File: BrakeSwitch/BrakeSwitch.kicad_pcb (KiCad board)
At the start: 2 copper layers, 82.3 x 59.8 mm, 31 parts, among them J1 12V_in, J2 LightPlug, J2 Signal_Breakout, J3 5V_out, J4 Front_Loop, J5 Rear_Loop, J6 12V_Out, J7 Front_Brake_Switch, J8 Rear_Brake_Switch, J9 Light_In, Q1 NMOS, SW1 AT SW-R2-2B-F-1-0, U1 XL1509-5.0, U2 LMV321, U3 LMV321

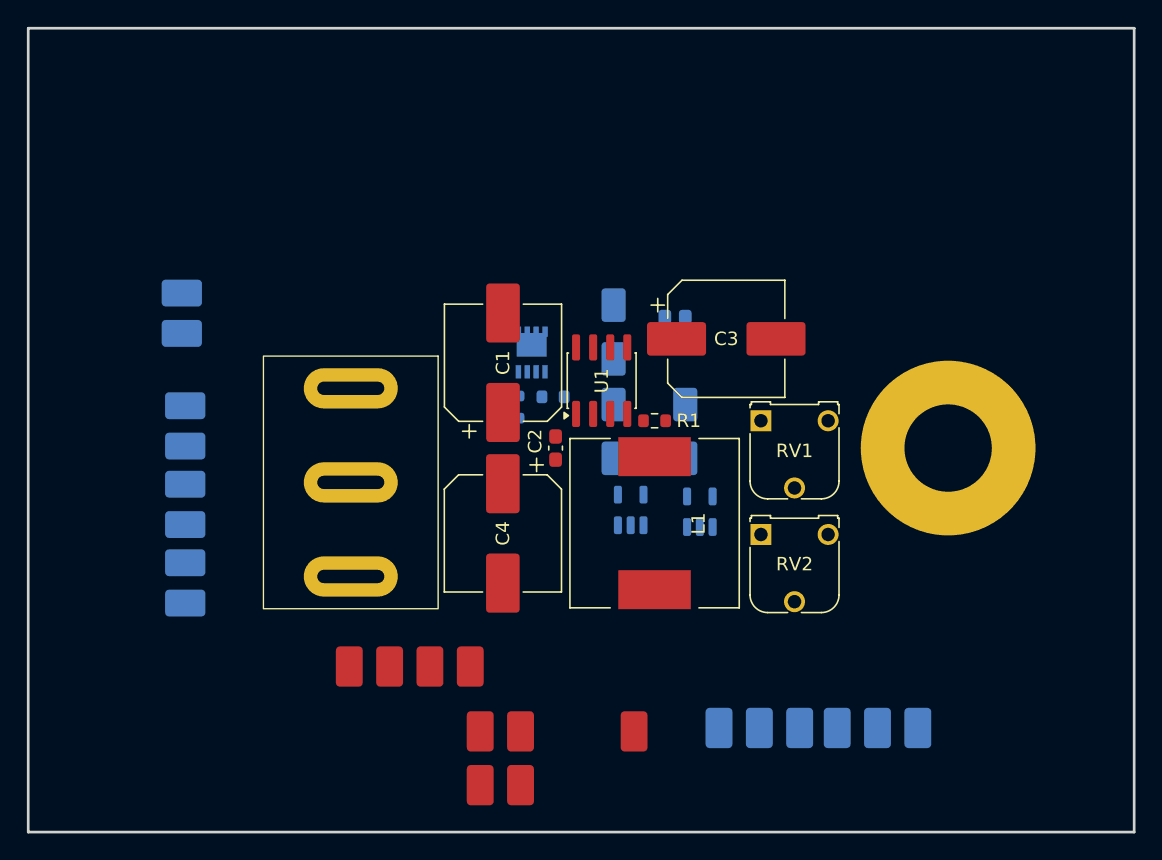
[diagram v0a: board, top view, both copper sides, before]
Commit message: Layout doneish
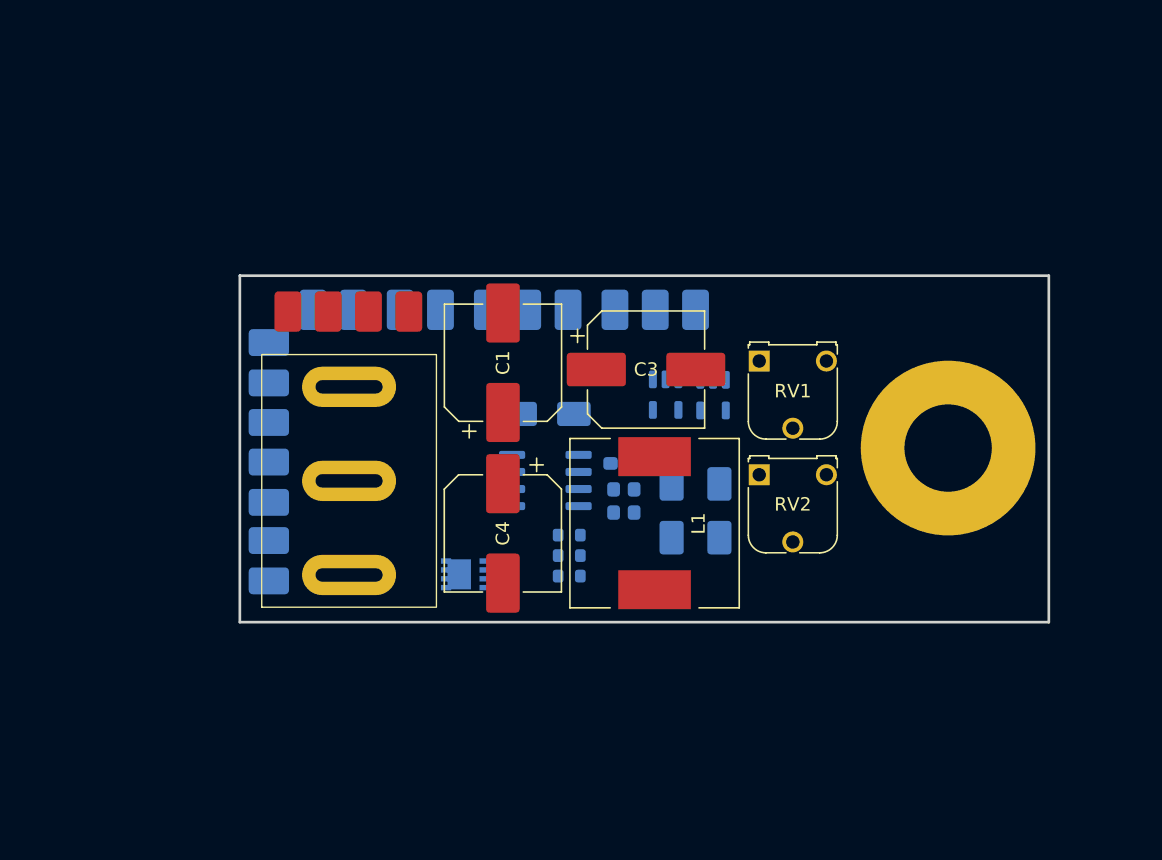
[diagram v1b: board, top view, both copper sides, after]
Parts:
- removed the J2 at (35.7, 40.8)
- C2, J7, J8, J9, R1, U1: moved to B.Cu
- moved J4 40.6 mm to (61.4, 40.5)
- moved J8 37.5 mm to (46.9, 40.5), turned to 180 degrees
- moved J9 35.6 mm to (42.2, 48.9), turned to 90 degrees
- moved J5 32.1 mm to (70.9, 40.5)
- moved J7 31.9 mm to (53.4, 40.5), turned to 180 degrees
- moved J2 26.8 mm to (48.1, 40.6)
- moved Q1 17.2 mm to (56.9, 60.2), turned to 180 degrees
- moved C6 13.9 mm to (67.8, 54.7)
- moved R5 13.1 mm to (64.5, 60.3), turned to 0 degrees
- moved C5 13.0 mm to (69.3, 54.7)
- moved R4 11.9 mm to (64.5, 58.8)
- moved R1 10.6 mm to (64.5, 57.3), turned to 180 degrees
- moved U3 10.5 mm to (75.2, 46.9), turned to -90 degrees
- moved D3 9.84 mm to (75.7, 55.5), turned to 90 degrees
- moved U2 9.08 mm to (71.7, 46.8), turned to -90 degrees
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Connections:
- net SwitchF- renamed GND
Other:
- board size 82.3 x 59.8 mm -> 60.2 x 25.8 mm

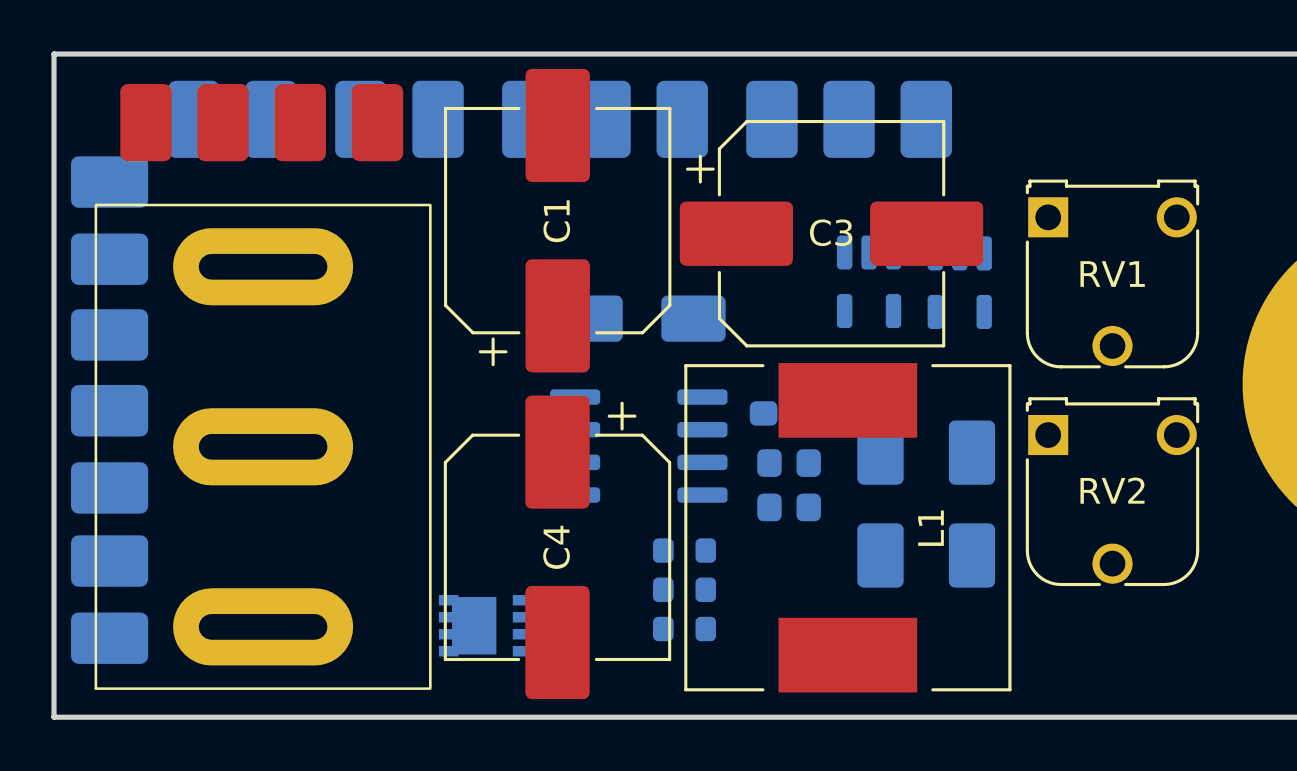
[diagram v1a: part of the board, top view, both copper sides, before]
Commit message: Starting traces
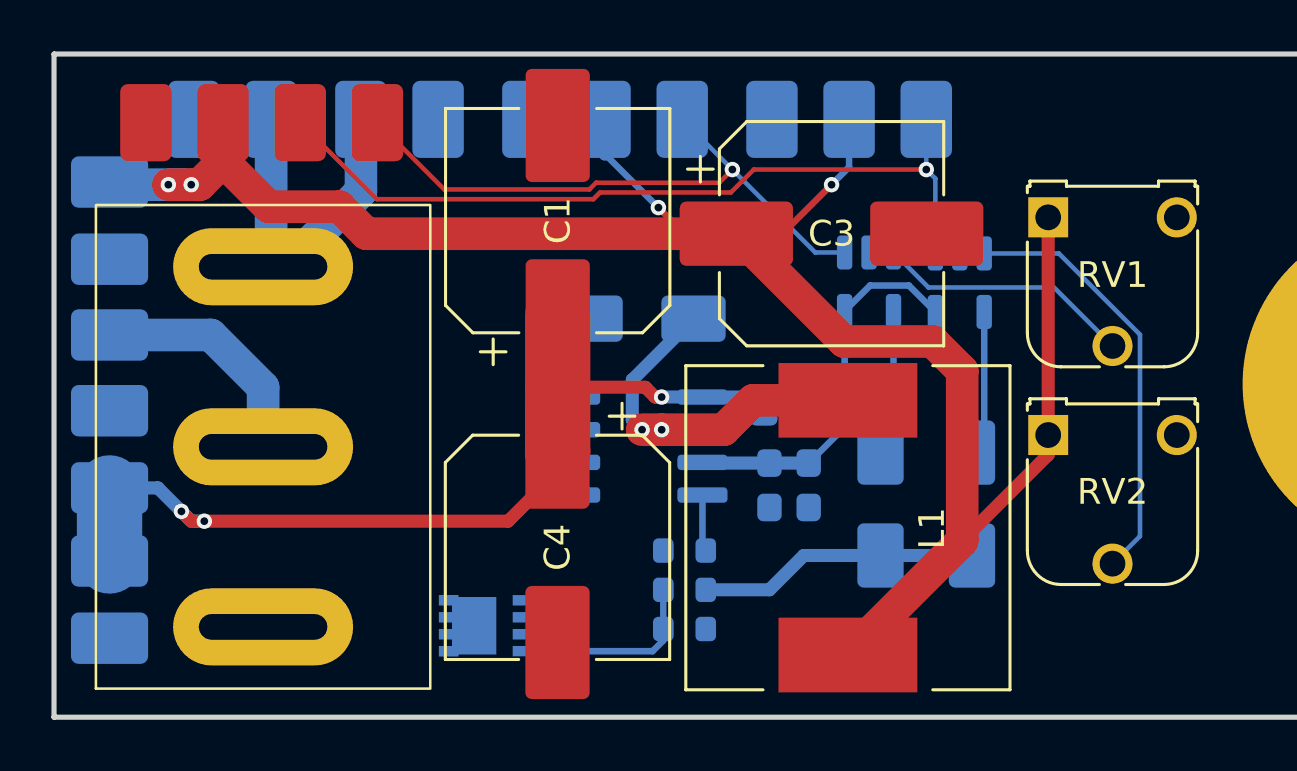
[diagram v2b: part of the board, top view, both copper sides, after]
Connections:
- J6 pad 1: 12V_out -> 12V
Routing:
- net 5V: track 0.00 -> 96.2 mm, vias 0 -> 4
- net 12V: track 0.00 -> 37.1 mm, vias 0 -> 3
- net RearLoop: track 0.00 -> 31.4 mm, vias 0 -> 1
- net FrontLoop: track 0.00 -> 23.7 mm, vias 0 -> 1
- net Net-(U3--): track 0.00 -> 16.7 mm
- net Net-(D1-K): track 0.00 -> 16.3 mm, vias 0 -> 2
- net SwitchF+: track 0.00 -> 13.7 mm
- net Net-(D2-K): track 0.00 -> 10.9 mm
- net Net-(U2--): track 0.00 -> 10.0 mm
- net Light In: track 0.00 -> 9.13 mm
- net Net-(Q1-G): track 0.00 -> 7.50 mm
- net Net-(D2-A): track 0.00 -> 5.71 mm
- net Net-(D3-A): track 0.00 -> 5.66 mm
- net Net-(U1-~{EN}): track 0.00 -> 2.21 mm
